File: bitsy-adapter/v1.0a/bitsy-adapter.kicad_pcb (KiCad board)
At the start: 2 copper layers, 49.5 x 36.8 mm, 17 parts, among them J1 PMOD1A, J2 PMOD1A, J3 PMOD1A, J4 5V AUX, J5 5V AUX, J6 5V AUX

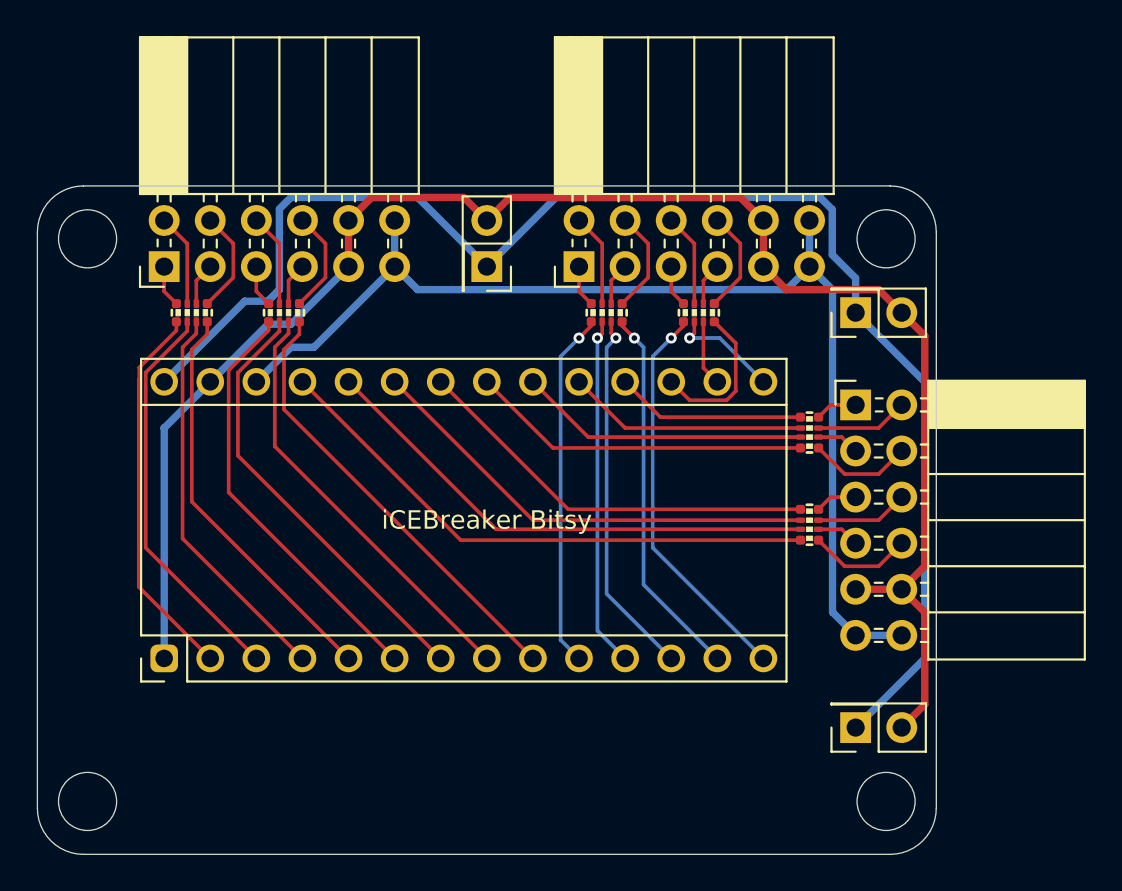
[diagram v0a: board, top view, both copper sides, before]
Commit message: Finish bitsy-adapter v1.0a
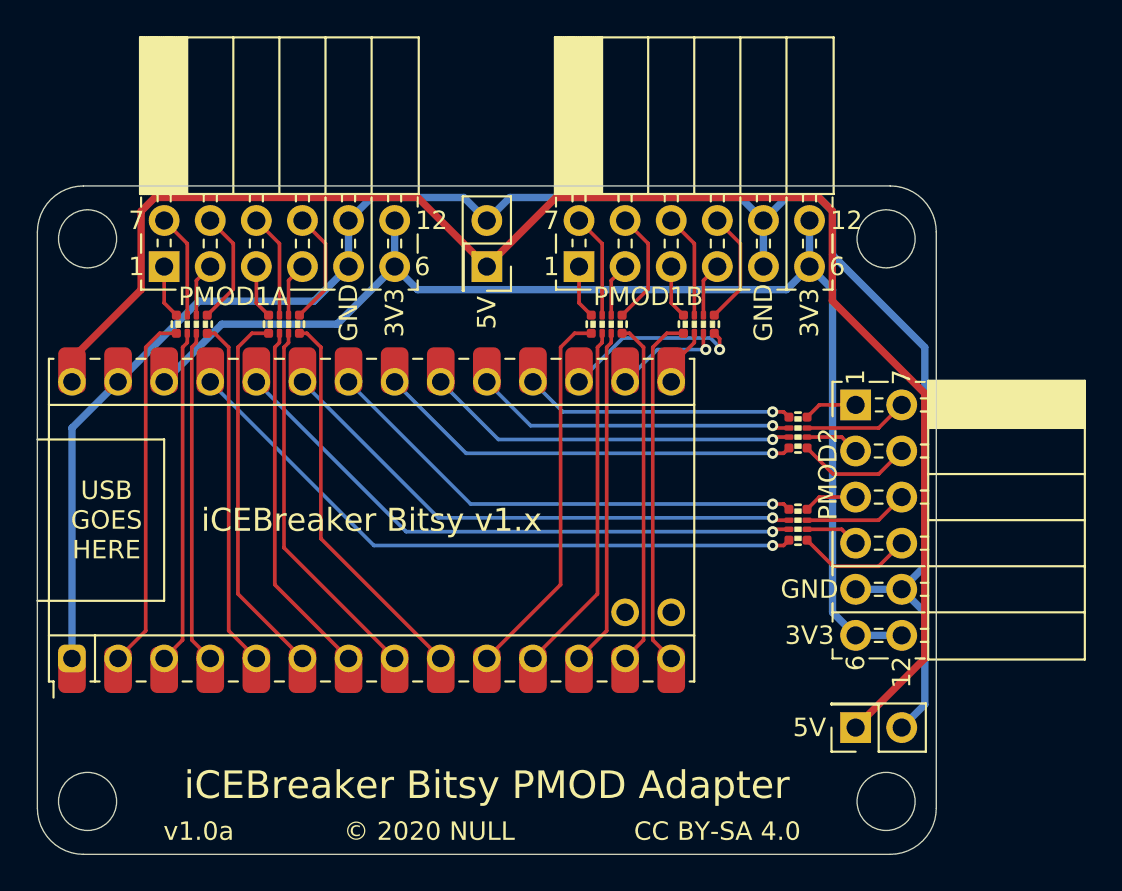
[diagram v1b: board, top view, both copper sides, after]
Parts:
- removed the J5 at (160.0, 102.9)
- added J6: IO3, pkl_pin_headers:Pin_Header_Straight_Round_1x01, F.Cu at (147.3, 119.4)
- added J7: IO2, pkl_pin_headers:Pin_Header_Straight_Round_1x01, F.Cu at (149.9, 119.4)
- added LOGO1: 1BitSquared, pkl_logos:null_Logo_SilkS_4mm, B.Cu at (139.7, 130.2)
- moved A1 5.08 mm to (133.3, 114.3)
- moved R1 0.63 mm to (123.4, 103.5)
- moved R2 0.63 mm to (128.5, 103.5)
- moved R3 0.63 mm to (146.3, 103.5)
- moved R4 0.63 mm to (151.4, 103.5)
- moved R5 0.63 mm to (156.8, 109.5)
- moved R6 0.63 mm to (156.8, 114.6)
- renumbered J6 to J5
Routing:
- net GND: track 92.8 -> 101.0 mm
- net +5V: track 79.3 -> 85.0 mm
- net +3V3: track 63.2 -> 68.2 mm
- net /P2_10: track 31.1 -> 35.7 mm, vias 0 -> 1
- net /P2_8: track 18.8 -> 23.5 mm, vias 0 -> 1
- net /P2_4: track 28.3 -> 32.8 mm, vias 0 -> 1
- net /P2_2: track 16.0 -> 20.6 mm, vias 0 -> 1
- net /P2_7: track 13.3 -> 17.7 mm, vias 0 -> 1
- net /P2_9: track 25.5 -> 30.0 mm, vias 0 -> 1
- net /P2_1: track 10.5 -> 14.9 mm, vias 0 -> 1
- net /P2_3: track 22.7 -> 27.2 mm, vias 0 -> 1
- net /P1A9: track 24.1 -> 19.7 mm
- net /P1A7: track 22.0 -> 18.4 mm
- net /P1B9: track 6.07 -> 2.57 mm, vias 1 -> 0
- net /P1A8: track 22.5 -> 19.3 mm
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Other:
- board text added: ""5V" is connected to VIN on the Bitsy, which is in turn jumpered to VUSB"
- board text added: "1"
- board text added: "12"
- board text added: "3V3"
- board text added: "5V"
- board text added: "6"
- board text added: "7"
- board text added: "CC BY-SA 4.0"
- board text added: "GND"
- board text added: "IO2"
- board text added: "IO3"
- board text added: "P1A1"
- board text added: "P1A10"
- board text added: "P1A2"
- board text added: "P1A3"
- board text added: "P1A4"
- board text added: "P1A7"
- board text added: "P1A8"
- board text added: "P1A9"
- board text added: "P1B1"
- board text added: "P1B10"
- board text added: "P1B2"
- board text added: "P1B3"
- board text added: "P1B4"
- board text added: "P1B7"
- board text added: "P1B8"
- board text added: "P1B9"
- board text added: "P2_1"
- board text added: "P2_10"
- board text added: "P2_2"
- board text added: "P2_3"
- board text added: "P2_4"
- board text added: "P2_7"
- board text added: "P2_8"
- board text added: "P2_9"
- board text added: "PMOD1A"
- board text added: "PMOD1B"
- board text added: "PMOD2"
- board text added: "USB GOES HERE"
- board text added: "VIN"
- board text added: "iCEBreaker Bitsy PMOD Adapter"
- board text added: "iCEBreaker Bitsy PMOD Adapter v1.0a"
- board text added: "iCEBreaker Bitsy v1.x"
- board text added: "v1.0a"
- board text added: "© 2020 NULL"
- board text added: "© 2020 NULL CC BY-SA 4.0"
- board text removed: "iCEBreaker Bitsy"
